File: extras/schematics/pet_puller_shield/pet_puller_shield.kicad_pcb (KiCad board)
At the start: 2 copper layers, 75.4 x 53.8 mm, 19 parts, among them J1 Jack-DC, J2 Conn_01x02, J3 Conn_01x02, J4 Conn_01x02, J5 Conn_01x04, Q1 IRF540N, U1 LM317_TO-220, U2 MX1508_module

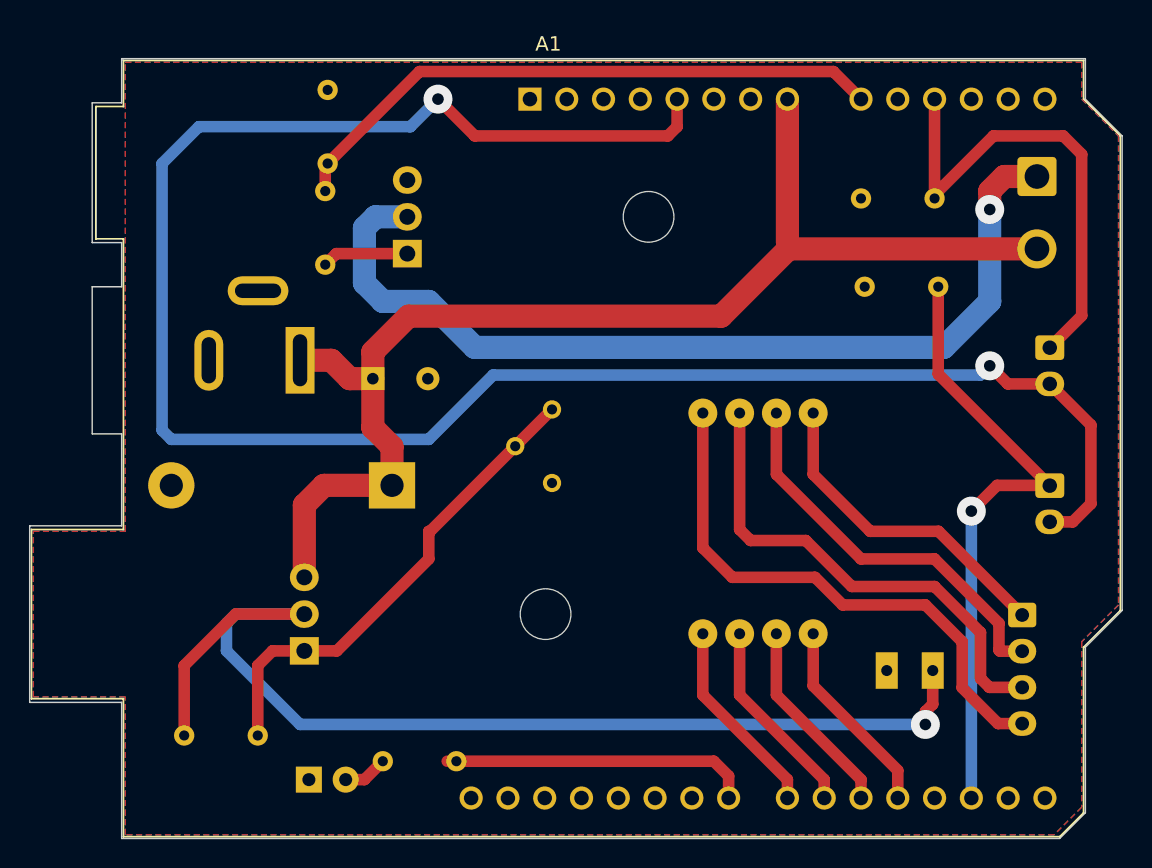
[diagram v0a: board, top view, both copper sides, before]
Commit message: Update schematics
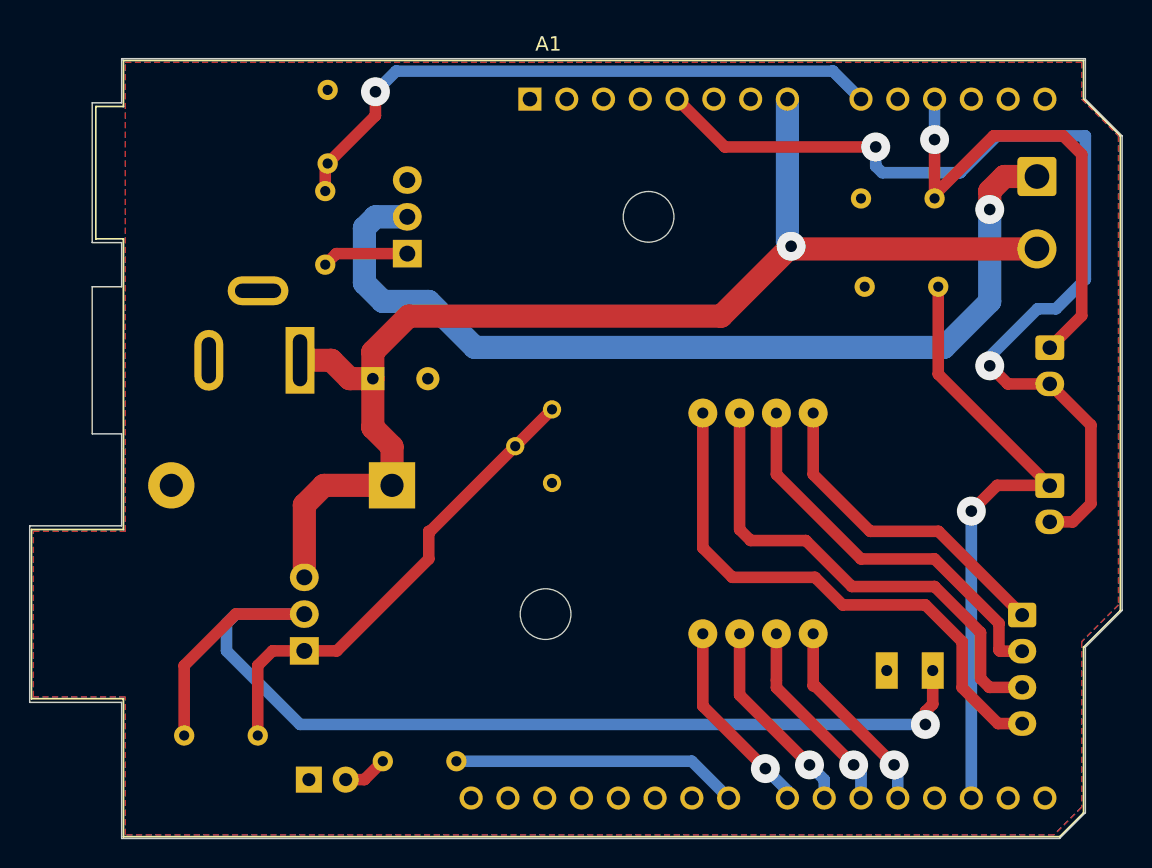
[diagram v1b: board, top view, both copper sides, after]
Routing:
- net +5V: track 136.0 -> 69.0 mm
- net LED: track 21.4 -> 19.9 mm
- net HOTEND: track 42.2 -> 43.2 mm, vias 0 -> 1
- net M0: vias 0 -> 1
- net M1: vias 0 -> 1
- net M2: vias 0 -> 1
- net THERMISTOR: vias 0 -> 1
- net M3: vias 0 -> 1
- net +12V: vias 0 -> 1
